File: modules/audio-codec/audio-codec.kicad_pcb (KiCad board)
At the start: 2 copper layers, 22 x 27.9 mm, 24 parts, among them U1 TLV320AIC3110IRHBR, U2 ADP5301ACBZ-1-R7

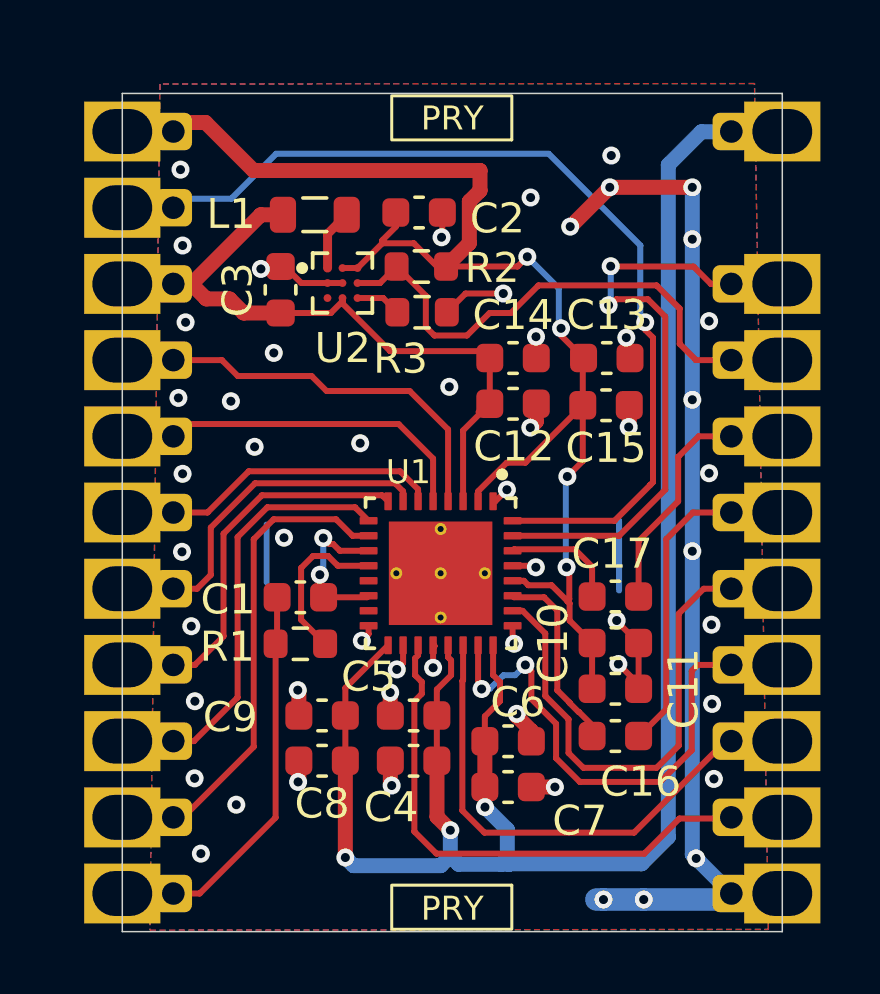
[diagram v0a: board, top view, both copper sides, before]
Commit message: Updating all modules
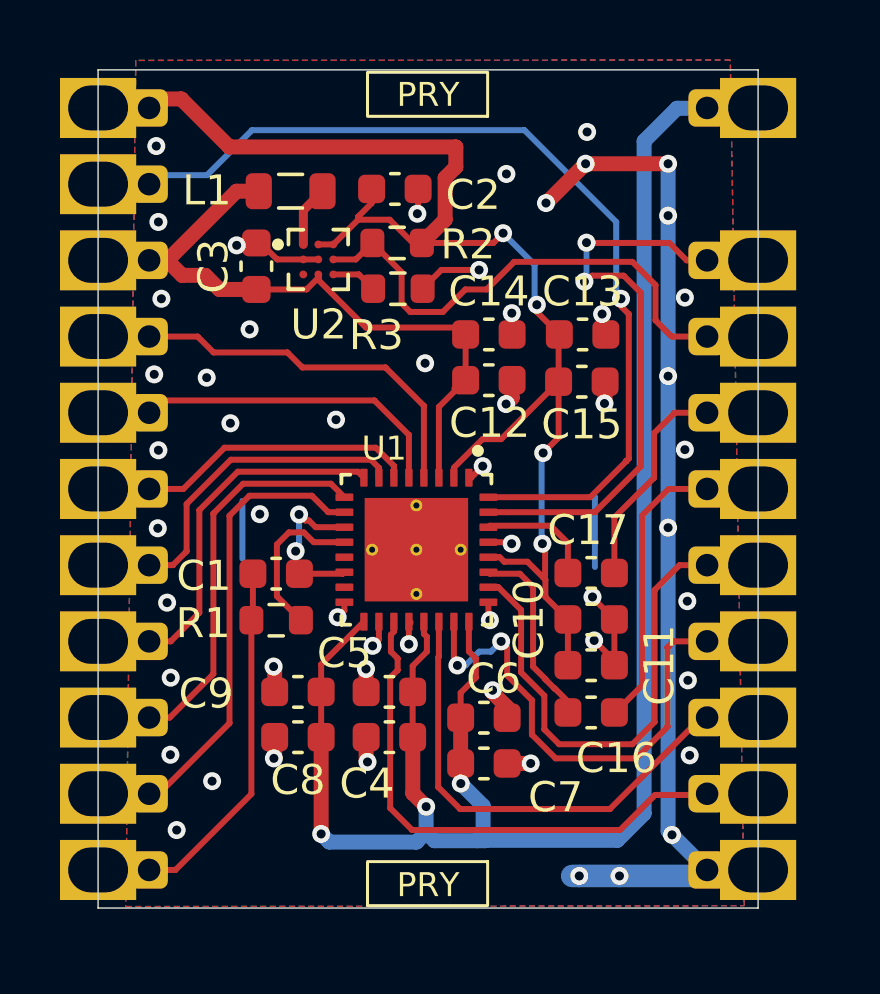
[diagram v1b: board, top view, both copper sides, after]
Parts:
- moved C13 1.13 mm to (88.8, 57.4)
- moved C14 1.13 mm to (85.7, 57.4)
- moved U2 1.13 mm to (80.0, 54.9)
- moved C1 1.13 mm to (78.6, 65.4)
- moved C10 1.13 mm to (89.1, 66.9)
- moved C11 1.13 mm to (89.1, 68.4)
- moved C12 1.13 mm to (85.7, 58.9)
- moved C15 1.13 mm to (88.8, 59.0)
- moved C16 1.13 mm to (89.1, 70.0)
- moved C17 1.13 mm to (89.1, 65.4)
- moved C3 1.13 mm to (78.0, 55.1)
- moved C6 1.13 mm to (85.6, 70.2)
- moved C7 1.13 mm to (85.6, 71.7)
- moved L1 1.13 mm to (79.1, 52.6)
- moved M1 1.13 mm to (83.7, 62.6)
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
